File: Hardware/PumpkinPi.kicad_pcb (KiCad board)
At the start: 4 copper layers, 19.4 x 29.7 mm, 18 parts, among them J2 Conn_01x04, J3 0475710001, J4 Conn_01x05, J5 Conn_01x05, J6 Conn_01x05, U1 F1C100s, U2 TPS717xx, U3 TPS717xx, U4 TPS717xx, Y1 Crystal_GND24

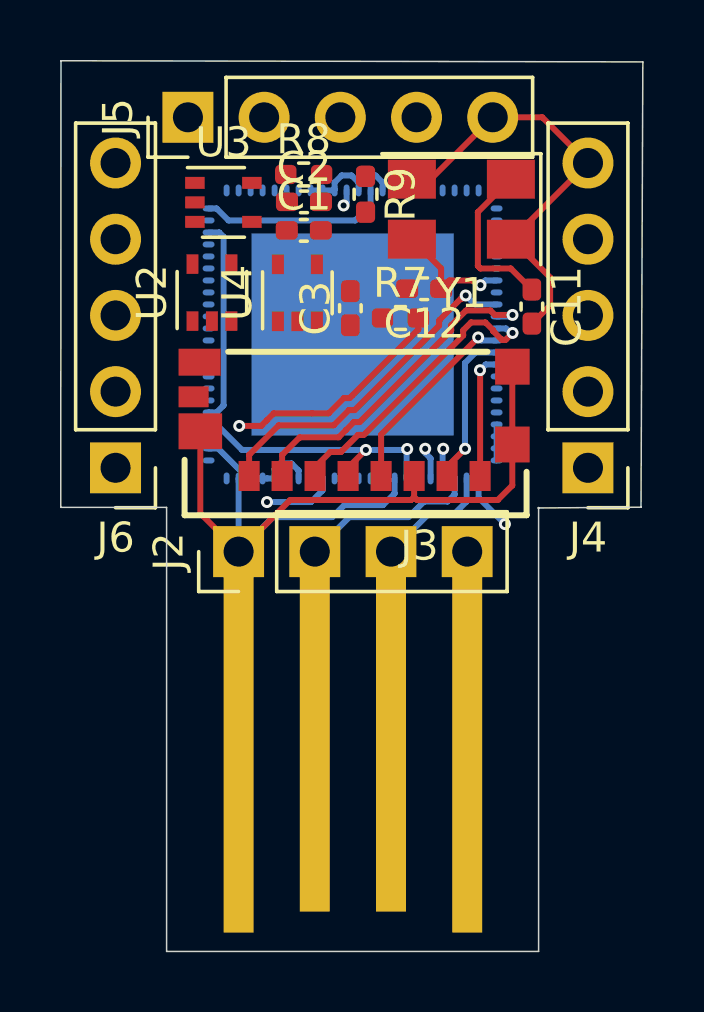
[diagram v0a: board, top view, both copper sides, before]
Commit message: routing done
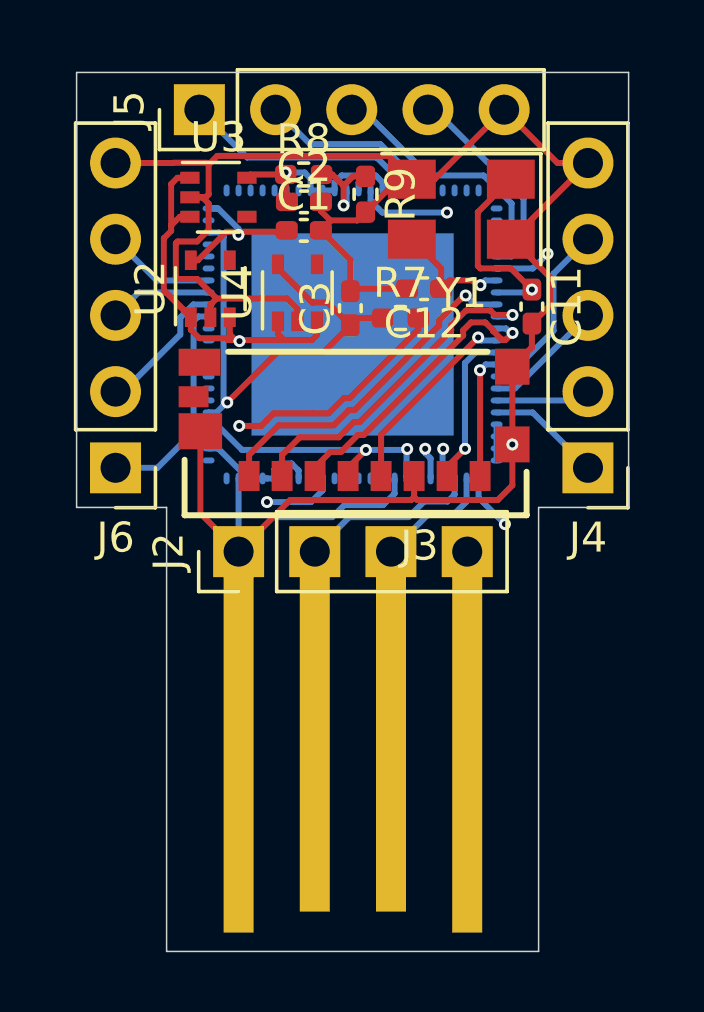
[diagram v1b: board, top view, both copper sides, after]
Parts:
- moved J5 0.46 mm to (101.1, 86.7)
- moved U3 0.24 mm to (101.7, 89.7)
- moved U2 0.14 mm to (101.5, 92.7)
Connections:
- J5 pad 3: /RX -> /TX
- J5 pad 4: /TX -> /RX
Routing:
- net GND: track 48.7 -> 82.4 mm, vias 0 -> 1
- net +3V3: track 18.2 -> 43.8 mm, vias 3 -> 5
- net /USB_VBUS: track 0.00 -> 24.6 mm, vias 0 -> 1
- net +1V1: track 7.33 -> 24.9 mm, vias 1 -> 3
- net +2V5: track 5.98 -> 22.1 mm, vias 1 -> 2
- net /TX: track 0.00 -> 8.39 mm
- net /SDA: track 0.00 -> 7.92 mm
- net /PD7: track 0.00 -> 7.35 mm
- net /RX: track 0.00 -> 7.01 mm
- net /SPI_CLK: track 0.00 -> 6.06 mm
- net /SCL: track 0.00 -> 5.88 mm
- net /PD8: track 0.00 -> 4.64 mm
- net /SPI_CS: track 0.00 -> 4.05 mm
- net /SPI_MOSI: track 0.00 -> 3.81 mm
- net /PD10: track 0.00 -> 3.67 mm
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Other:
- board size 19.4 x 29.7 mm -> 18.4 x 29.3 mm
